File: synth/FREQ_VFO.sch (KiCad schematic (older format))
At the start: 33 parts

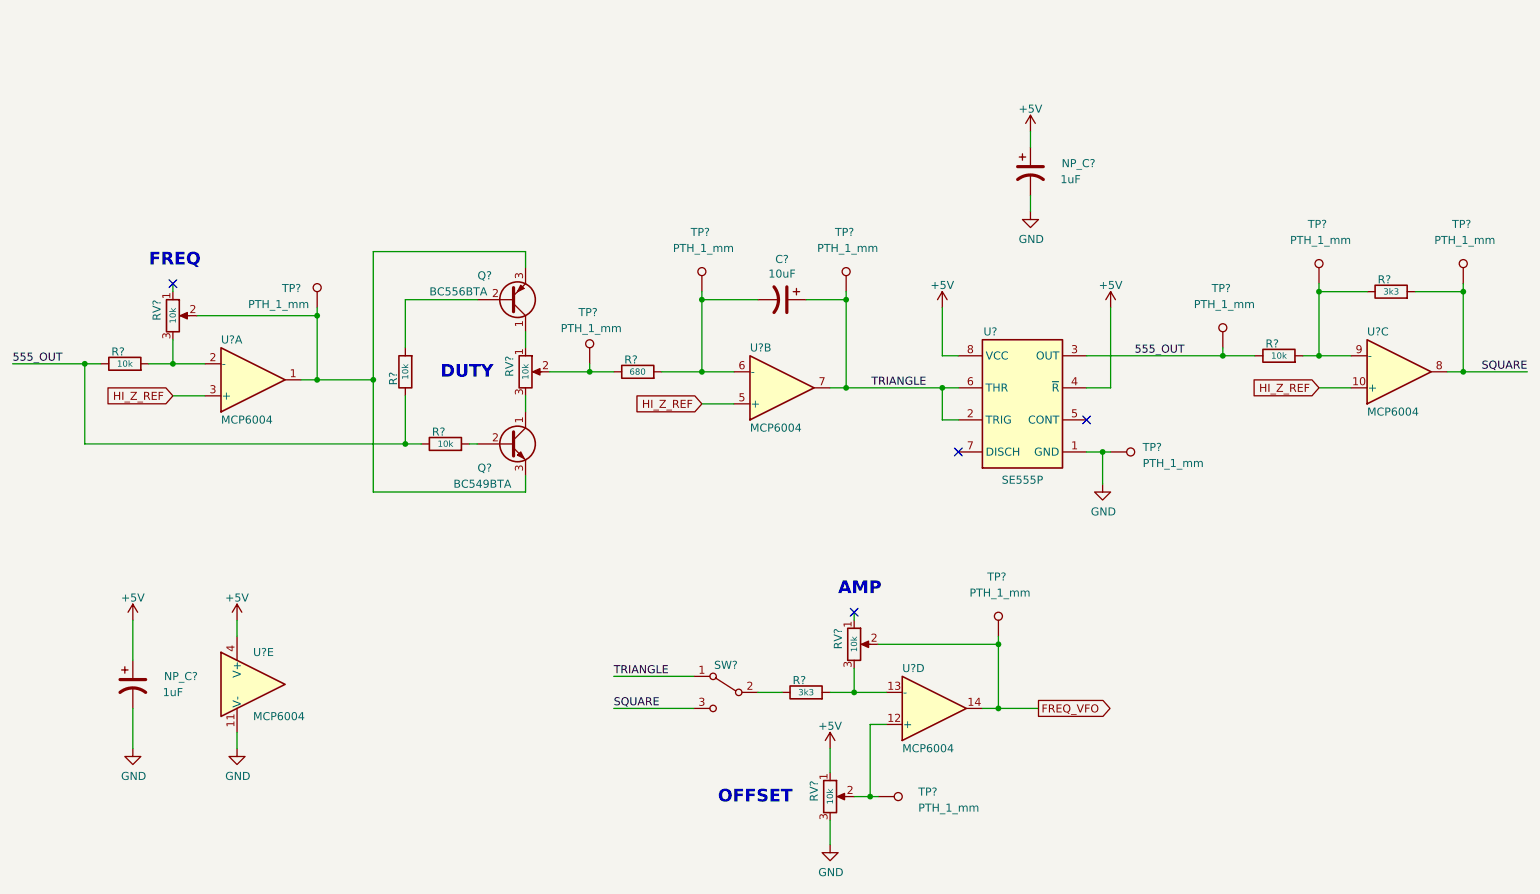
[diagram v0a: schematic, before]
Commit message: automated commit
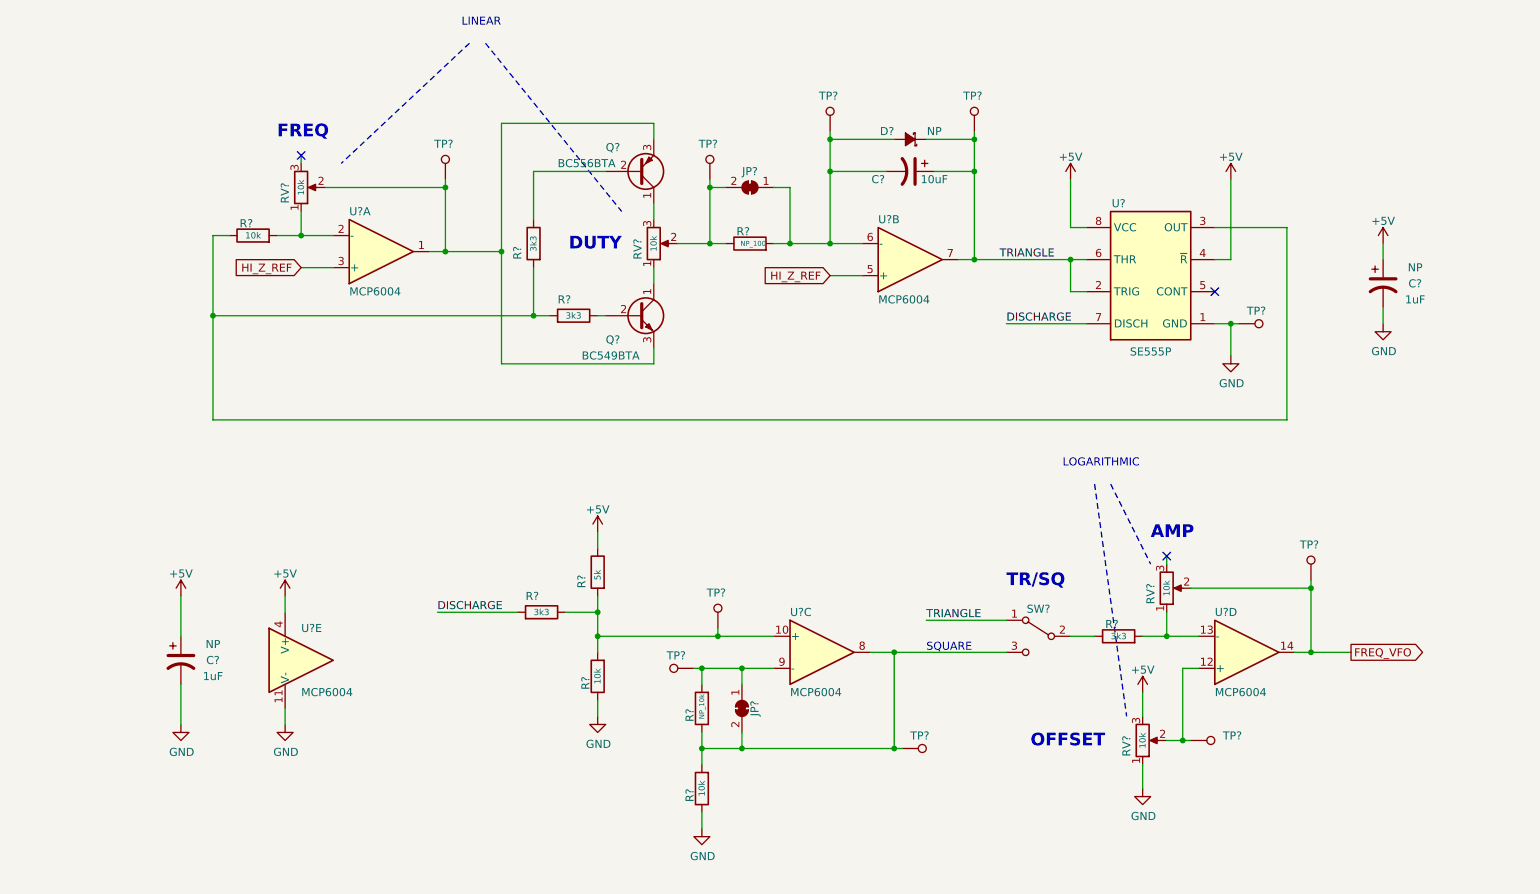
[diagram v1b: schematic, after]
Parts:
- removed R? (x3): 10k, symbol Device:R
- removed R?: 3k3, symbol Device:R
- removed TP? (x8): PTH_1_mm, TestPoint:TestPoint_THTPad_D2.0mm_Drill1.0mm, symbol custom:PTH_1_mm
- added D?: D_Schottky_Small_ALT, symbol Device:D_Schottky_Small_ALT
- added JP? (x2): SolderJumper_2_Bridged, symbol Jumper:SolderJumper_2_Bridged
- added R?: 5k, symbol Device:R
- added R? (x2): 10k, symbol Device:R
- added R? (x3): 3k3, symbol Device:R
- added R?: NP_10k, symbol Device:R
- added TP? (x8): PTH_1_mm, TestPoint:TestPoint_THTPad_D2.0mm_Drill1.0mm, symbol custom:PTH_1_mm
- C? (x2): renamed from NP_C?; NP (none) -> NP
- R?: value 680 -> NP_100
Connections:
- net +5V: now also RV?.3, R?.1; no longer RV?.1
- net FREQ_VFO: now also TP?.1
- net GND: now also RV?.1, R?.1, R?.1; no longer RV?.3
- net HI_Z_REF: no longer U?.10 (+)
- net TRIANGLE: now also D?.1 (K)
- net DISCHARGE: now reaches U?.7 (DISCH)
- net DISCHARGE: now also R?.2
- net at C?.2, R?.2, U?.6 (-): now also D?.2 (A), JP?.1 (A), TP?.1
- net at R?.1, RV?.2: now also JP?.2 (B), TP?.1
- net at R?.2, U?.2 (-): now also RV?.1; no longer RV?.3
- net at Q?.3 (E), Q?.3 (E), RV?.2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: now also TP?.1
- net at Q?.2 (B): now also R?.1 (x2)
- net at U?.9 (-): now also JP?.1 (A), R?.2, TP?.1
- net at RV?.2, U?.12 (+): now also TP?.1
- net at R?.2, U?.13 (-): now also RV?.1; no longer RV?.3
- net at Q?.1 (C): now also RV?.1; no longer RV?.3
- net at Q?.1 (C): now also RV?.3; no longer RV?.1
- net 555_OUT: no longer names the net of R?.1, U?.3 (OUT)
- net 555_OUT: now also R?.2, R?.2
- net SQUARE: no longer names the net of SW?.3 (C), U?.8
- net SQUARE: now also JP?.2 (B), R?.1, R?.2, TP?.1
- new net: R?.1, R?.2, R?.2, TP?.1, U?.10 (+)
- no-connect marks 4 -> 3
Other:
- note added: "LINEAR"
- note added: "LOGARITHMIC"
- note added: "SQUARE"
- note added: "TR/SQ"
- moved on the sheet: C?, Q?, R?, RV?, SW?, TP?, U?, U?A, U?B, U?C, U?D, U?E
